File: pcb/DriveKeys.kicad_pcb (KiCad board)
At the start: 2 copper layers, 152.4 x 101.6 mm, 0 parts

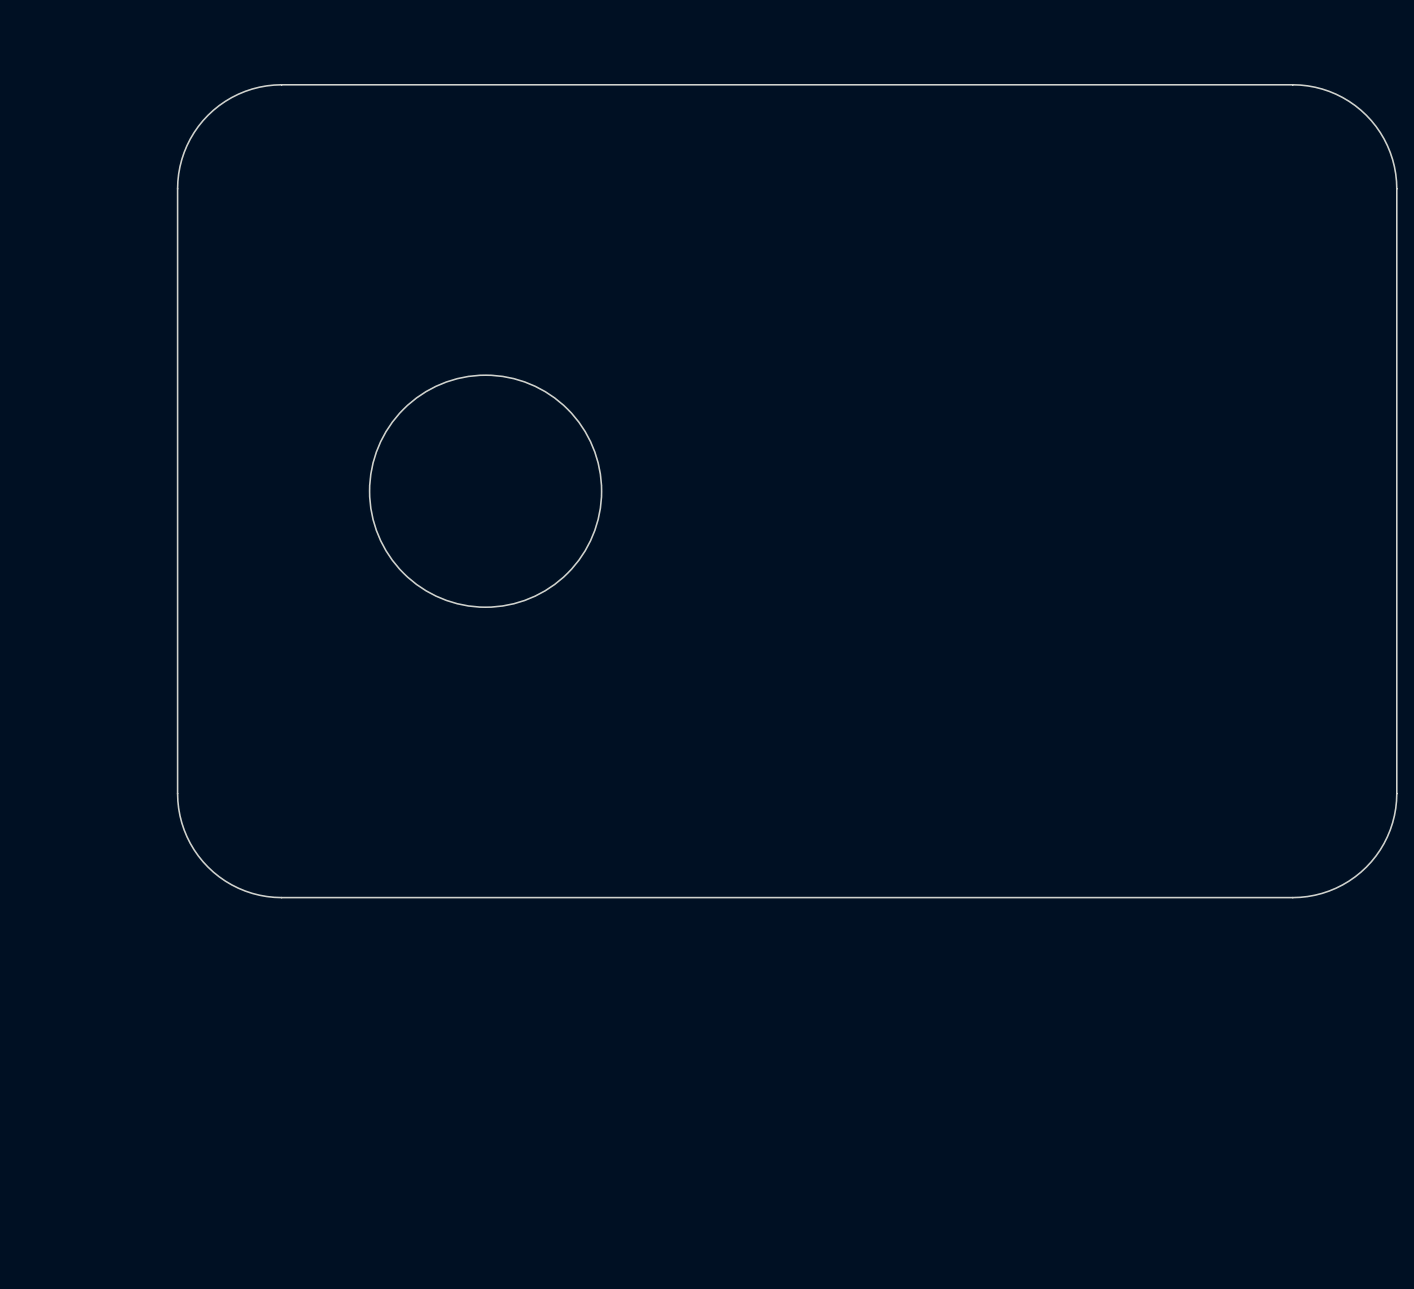
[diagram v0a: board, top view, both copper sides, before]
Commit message: feat: laying out design
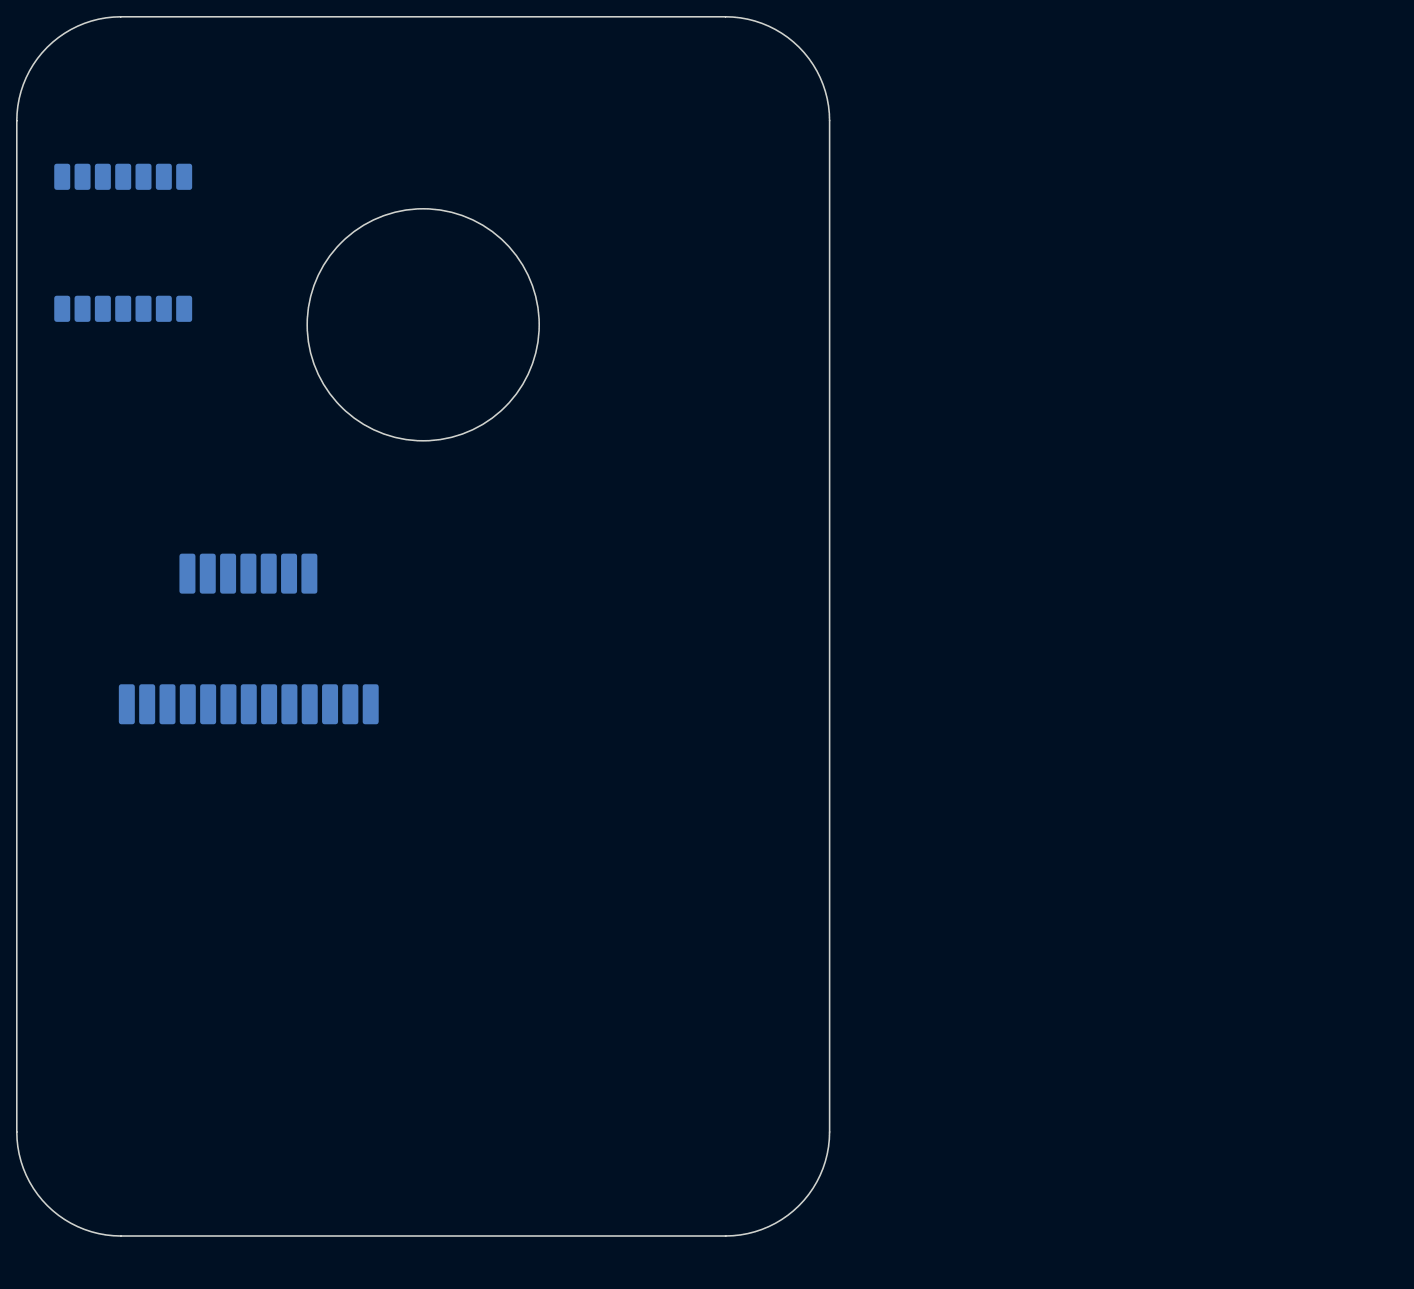
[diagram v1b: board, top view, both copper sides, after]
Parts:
- added QT Py Pad: QT Py Pad, Library:QT Py Pad, B.Cu at (63.7, 55.3)
- added REF**: Adafruit MPR121, Library:Adafruit MPR121, B.Cu at (63.0, 106.5)
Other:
- board size 152.4 x 101.6 mm -> 101.6 x 152.4 mm

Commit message: wip: setting up touchpad
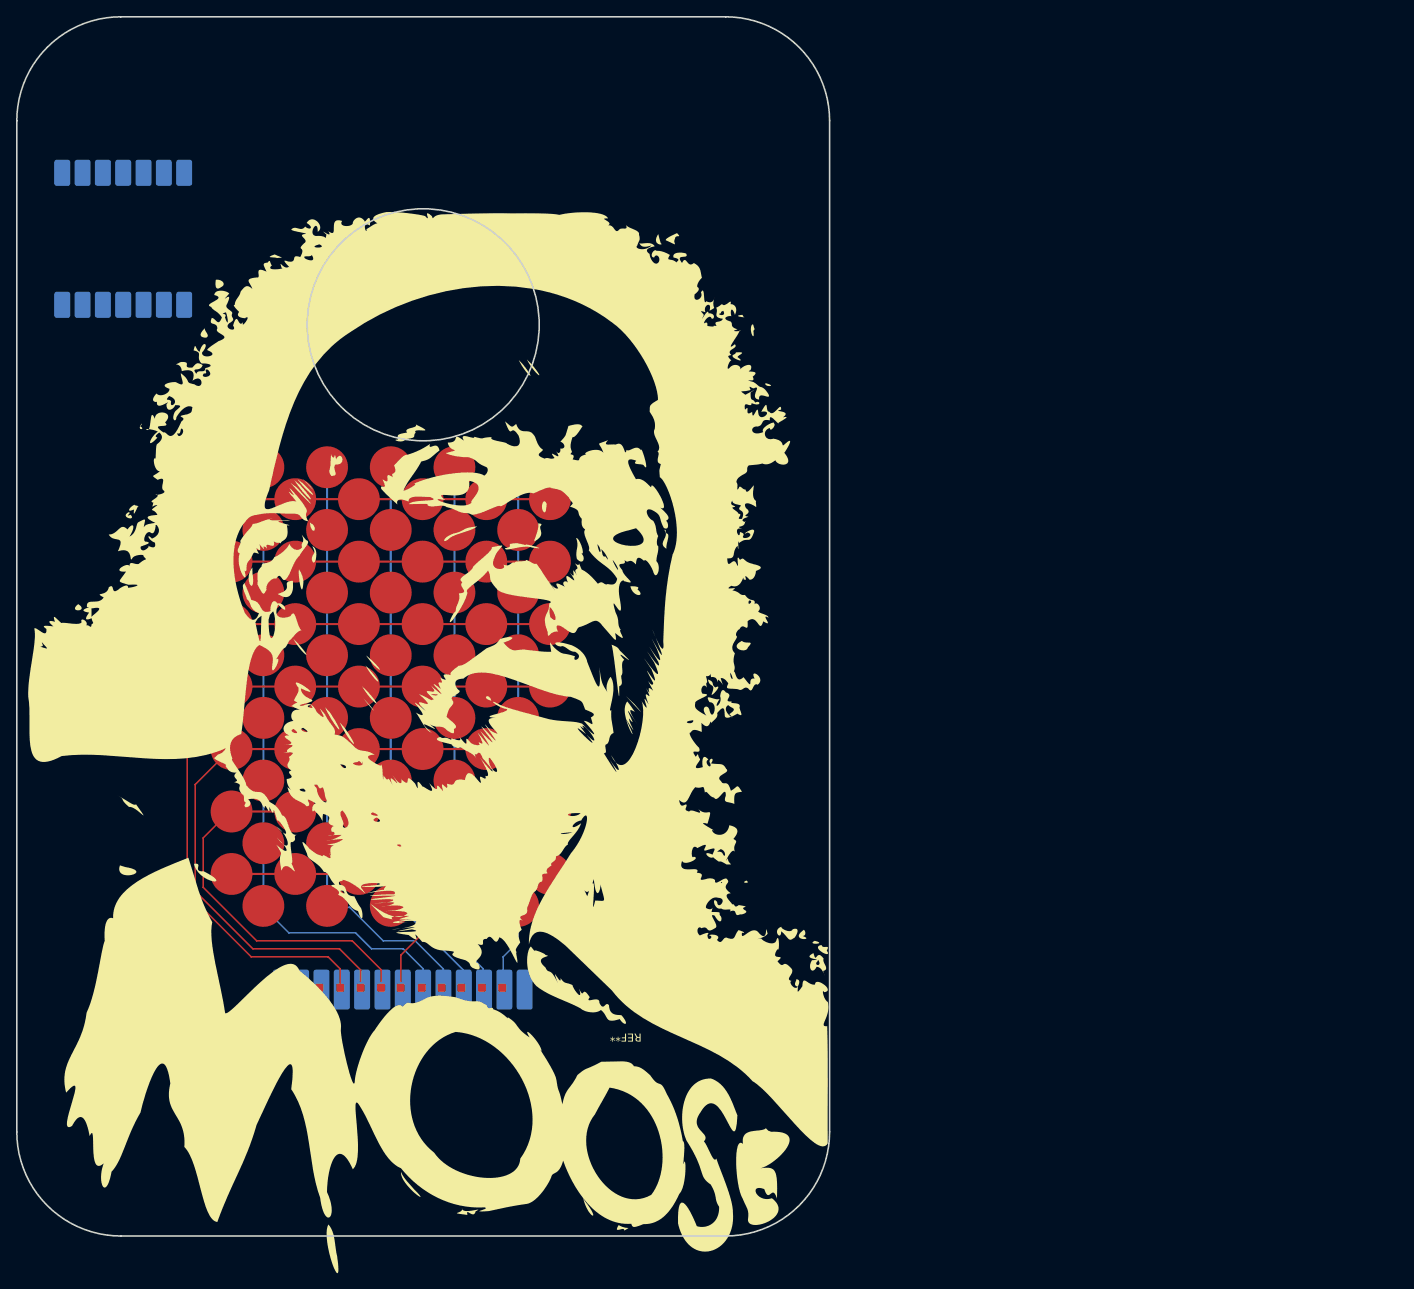
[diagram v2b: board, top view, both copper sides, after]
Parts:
- added REF**: Touchpad, Library:Touchpad, F.Cu at (127.3, 154.6)
- moved REF** 40.5 mm to (82.2, 142.2)
- moved QT Py Pad 0.50 mm to (63.7, 54.8)
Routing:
- net (no net): track 0.00 -> 237.0 mm
